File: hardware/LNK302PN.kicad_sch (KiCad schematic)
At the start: 7 parts, among them J101 AC, J102 PWM, J103 380OUT, J104 380_BP2876D, J105 LOAD, J107 3V3, J108 380_LNK302PN

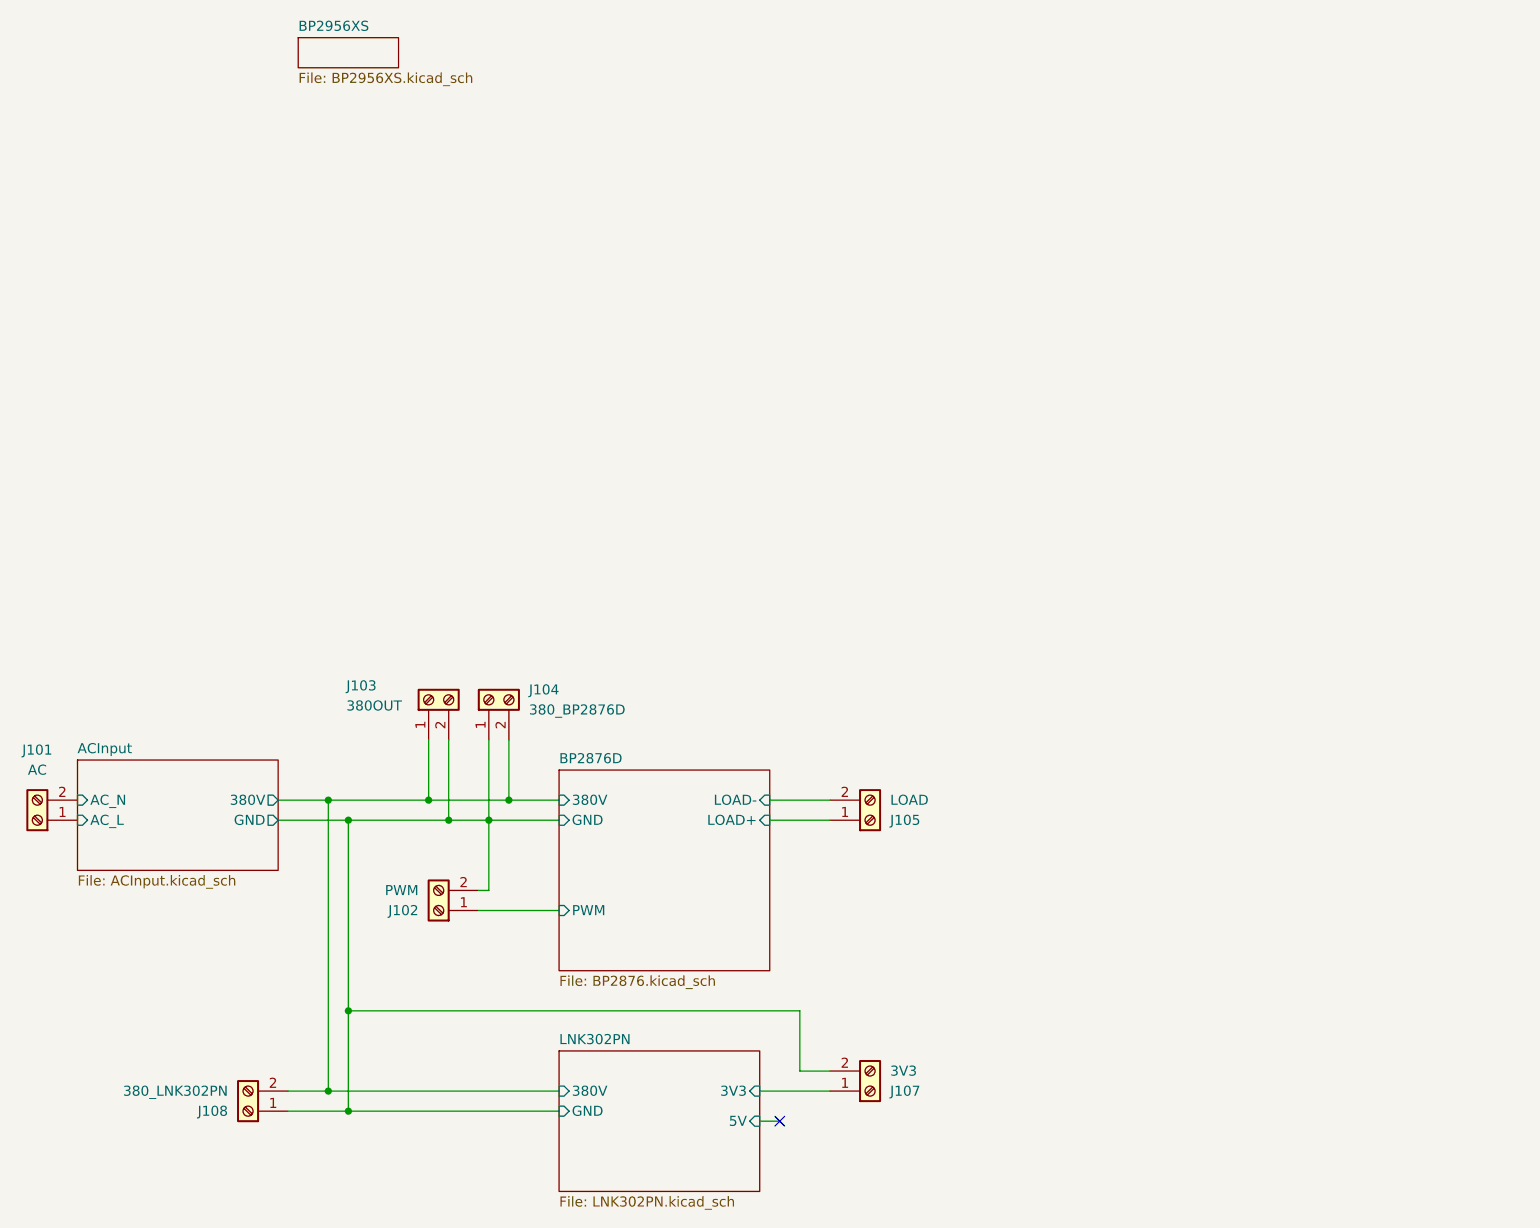
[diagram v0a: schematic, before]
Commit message: LNK302PN
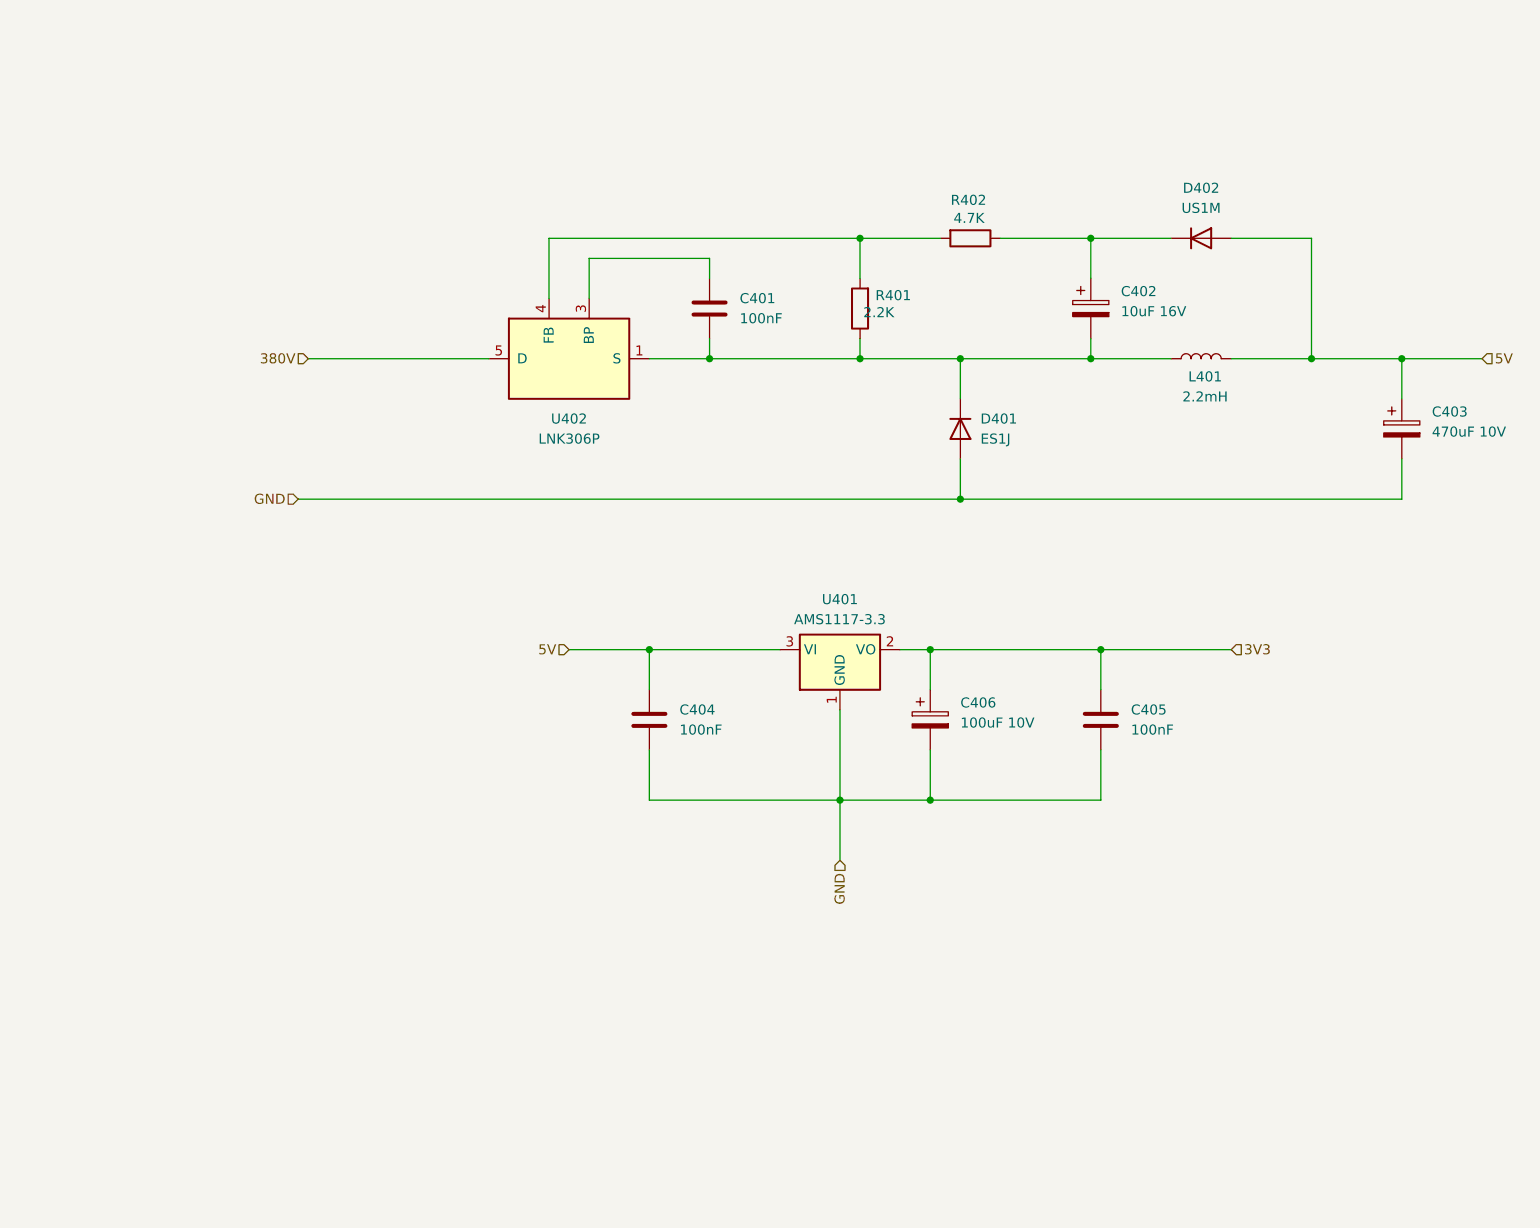
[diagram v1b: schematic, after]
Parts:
- removed J101: AC, TerminalBlock_Phoenix:TerminalBlock_Phoenix_MKDS-1,5-2-5.08_1x02_P5.08mm_Horizontal, symbol Connector:Screw_Terminal_01x02
- removed J102: PWM, TerminalBlock_Phoenix:TerminalBlock_Phoenix_MKDS-1-2-3.81_1x02_P3.81mm_Horizontal, symbol Connector:Screw_Terminal_01x02
- removed J103: 380OUT, TerminalBlock_Phoenix:TerminalBlock_Phoenix_MKDS-1,5-2-5.08_1x02_P5.08mm_Horizontal, symbol Connector:Screw_Terminal_01x02
- removed J104: 380_BP2876D, TerminalBlock_Phoenix:TerminalBlock_Phoenix_MKDS-1,5-2-5.08_1x02_P5.08mm_Horizontal, symbol Connector:Screw_Terminal_01x02
- removed J105: LOAD, TerminalBlock_Phoenix:TerminalBlock_Phoenix_MKDS-1,5-2-5.08_1x02_P5.08mm_Horizontal, symbol Connector:Screw_Terminal_01x02
- removed J107: 3V3, TerminalBlock_Phoenix:TerminalBlock_Phoenix_MKDS-1,5-2-5.08_1x02_P5.08mm_Horizontal, symbol Connector:Screw_Terminal_01x02
- removed J108: 380_LNK302PN, TerminalBlock_Phoenix:TerminalBlock_Phoenix_MKDS-1,5-2-5.08_1x02_P5.08mm_Horizontal, symbol Connector:Screw_Terminal_01x02
- added C401, C404, C405: 100nF, Capacitor_THT:C_Disc_D5.0mm_W2.5mm_P5.00mm, symbol Device:C
- added C402: 10uF 16V, Capacitor_THT:CP_Radial_D5.0mm_P2.50mm, symbol Device:C_Polarized
- added C403: 470uF 10V, Capacitor_THT:CP_Radial_D10.0mm_P5.00mm, symbol Device:C_Polarized
- added C406: 100uF 10V, Capacitor_THT:CP_Radial_D6.3mm_P2.50mm, symbol Device:C_Polarized
- added D401: ES1J, Diode_THT:D_DO-41_SOD81_P7.62mm_Horizontal, symbol Device:D
- added D402: US1M, Diode_THT:D_DO-41_SOD81_P7.62mm_Horizontal, symbol Device:D
- added L401: 2.2mH, Inductor_THT:L_Radial_D10.0mm_P5.00mm_Fastron_07M, symbol Device:L
- added R401: 2.2K, Resistor_THT:R_Axial_DIN0207_L6.3mm_D2.5mm_P7.62mm_Horizontal, symbol Device:R
- added R402: 4.7K, Resistor_THT:R_Axial_DIN0207_L6.3mm_D2.5mm_P7.62mm_Horizontal, symbol Device:R
- added U401: AMS1117-3.3, Package_TO_SOT_SMD:SOT-223-3_TabPin2, symbol Regulator_Linear:AMS1117-3.3
- added U402: LNK306P, Package_DIP:PowerIntegrations_PDIP-8B, symbol Regulator_Switching:LNK306P
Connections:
- new net: C402.1, D402.1 (K), R402.1
- new net: C401.1, C402.2, D401.1 (K), L401.1, R401.1, U402.1 (S), U402.2 (S), U402.7 (S), U402.8 (S)
- new net: C401.2, U402.3 (BP)
- new net: R401.2, R402.2, U402.4 (FB)
- new net 380V: U402.5 (D)
- new net 3V3: C405.2, C406.1, U401.2 (VO)
- new net 5V: C403.1, C404.2, D402.2 (A), L401.2, U401.3 (VI)
- new net GND: C403.2, C404.1, C405.1, C406.2, D401.2 (A), U401.1 (GND)
- no-connect marks 1 -> 0
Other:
- removed sheet ACInput
- removed sheet BP2876D
- removed sheet BP2956XS
- removed sheet LNK302PN
